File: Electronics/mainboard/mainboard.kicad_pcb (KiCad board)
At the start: 2 copper layers, 91.4 x 71.1 mm, 22 parts, among them J2 CONN_NIDEC_0, J3 CONN_NIDEC_1, J4 CONN_ESP32_L, J5 CONN_ESP32_R, J6 CONN_MPU6050, J7 Conn_Coaxial_Power, U3 LM7805_TO220

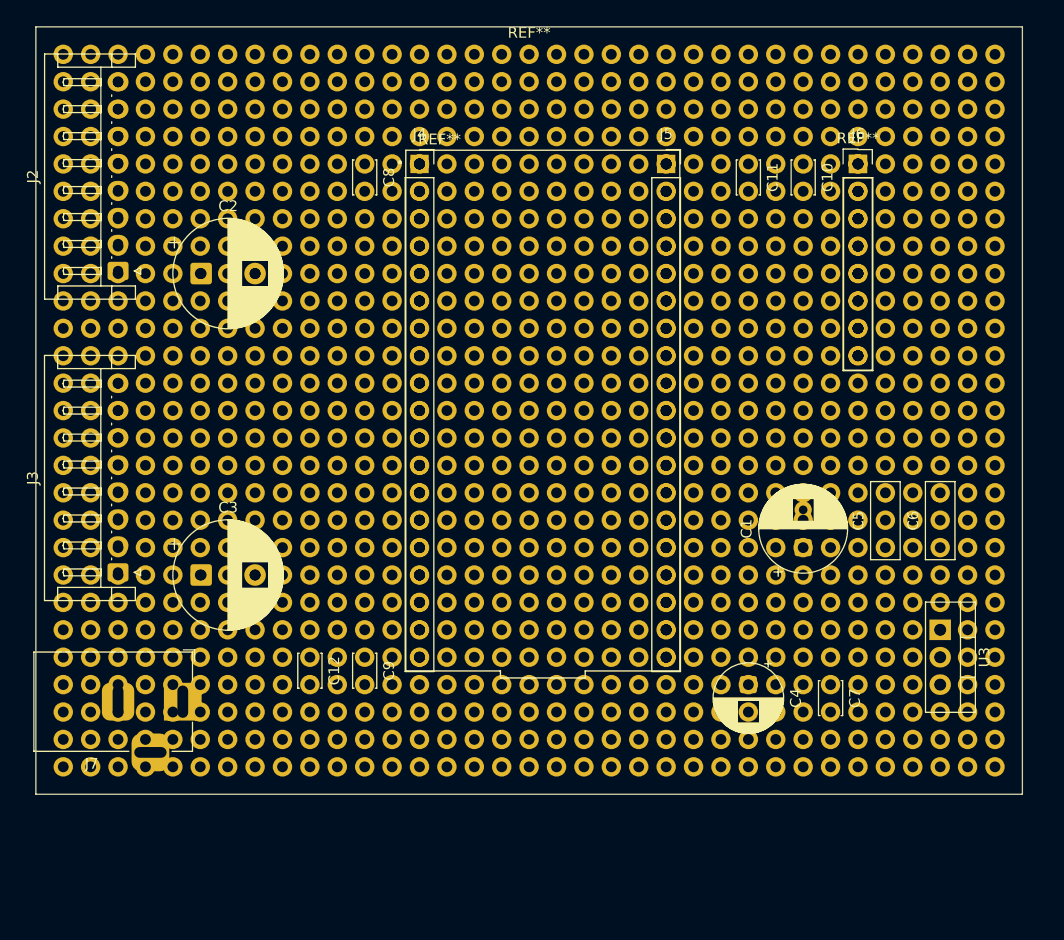
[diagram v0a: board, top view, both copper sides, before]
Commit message: improve PCB
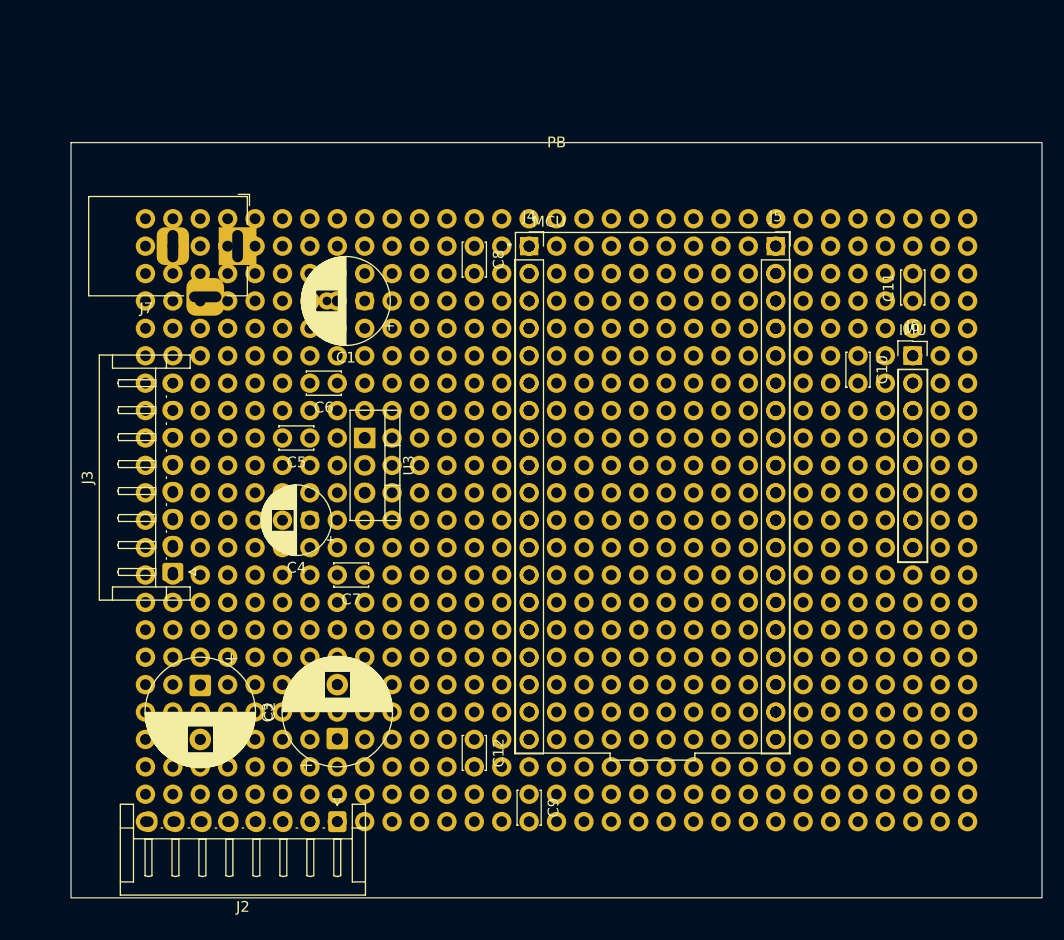
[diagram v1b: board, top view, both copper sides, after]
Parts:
- removed REF**: Perfboard_27x35_2.54mm, Perfboards:Perfboard_27x35_2.54mm
- added PB: Perfboard_90x70_2.54mm, Perfboards:Perfboard_90x70_2.54mm, F.Cu at (147.3, 101.6)
- C5, C6: footprint Capacitor_THT:C_Rect_L7.0mm_W2.5mm_P5.00mm -> Capacitor_THT:C_Disc_D3.0mm_W2.0mm_P2.50mm
- moved C6 57.9 mm to (127.0, 88.9), turned to 180 degrees
- moved U3 56.2 mm to (129.5, 94.0)
- moved J2 54.9 mm to (127.0, 129.5), turned to 180 degrees
- moved C5 54.3 mm to (124.5, 94.0), turned to 180 degrees
- moved C1 46.6 mm to (129.5, 81.3), turned to 180 degrees
- moved C2 44.9 mm to (127.0, 121.8), turned to 90 degrees
- moved C7 44.4 mm to (129.5, 106.7), turned to 180 degrees
- moved C4 43.4 mm to (124.5, 101.6), turned to 180 degrees
- moved J7 42.5 mm to (117.8, 76.2)
- moved C11 19.8 mm to (180.3, 81.3), turned to 90 degrees
- moved C9 19.8 mm to (144.8, 127.0)
- moved C10 18.5 mm to (175.3, 86.4)
- moved IMU 18.5 mm to (180.3, 86.4)
- moved J6 18.5 mm to (180.3, 86.4)
- moved C12 17.0 mm to (139.7, 121.9)
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- renumbered REF** to IMU, REF** to MCU
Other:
- board size 91.4 x 71.1 mm -> 90 x 70 mm
